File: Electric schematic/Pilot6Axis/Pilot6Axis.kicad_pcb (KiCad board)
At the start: 2 copper layers, 75.8 x 53.8 mm, 63 parts, among them IC1 ESP32-WROOM-32U, IC2 LM27313XMFX_NOPB, J1 BTN1, J10 Power switch, J11 TP4056, J12 OLED, J13 USB_C_Receptacle_USB2.0_16P, J14 BTN9, J15 BTN11, J16 BTN10, J2 BTN2, J3 BTN3, J4 BTN4, J5 BTN5, J6 BTN6, J7 BTN7, J8 BTN8, J9 BAT, Q1 Q_NPN_EBC, Q2 Q_NPN_EBC, SW1 SW_Push, SW2 SW_Push, U1 JOYSTICK1, U2 JOYSTICK2, U3 AMS1117-3.3, U4 USBLC6-2SC6, U5 CP2102N-Axx-xQFN28

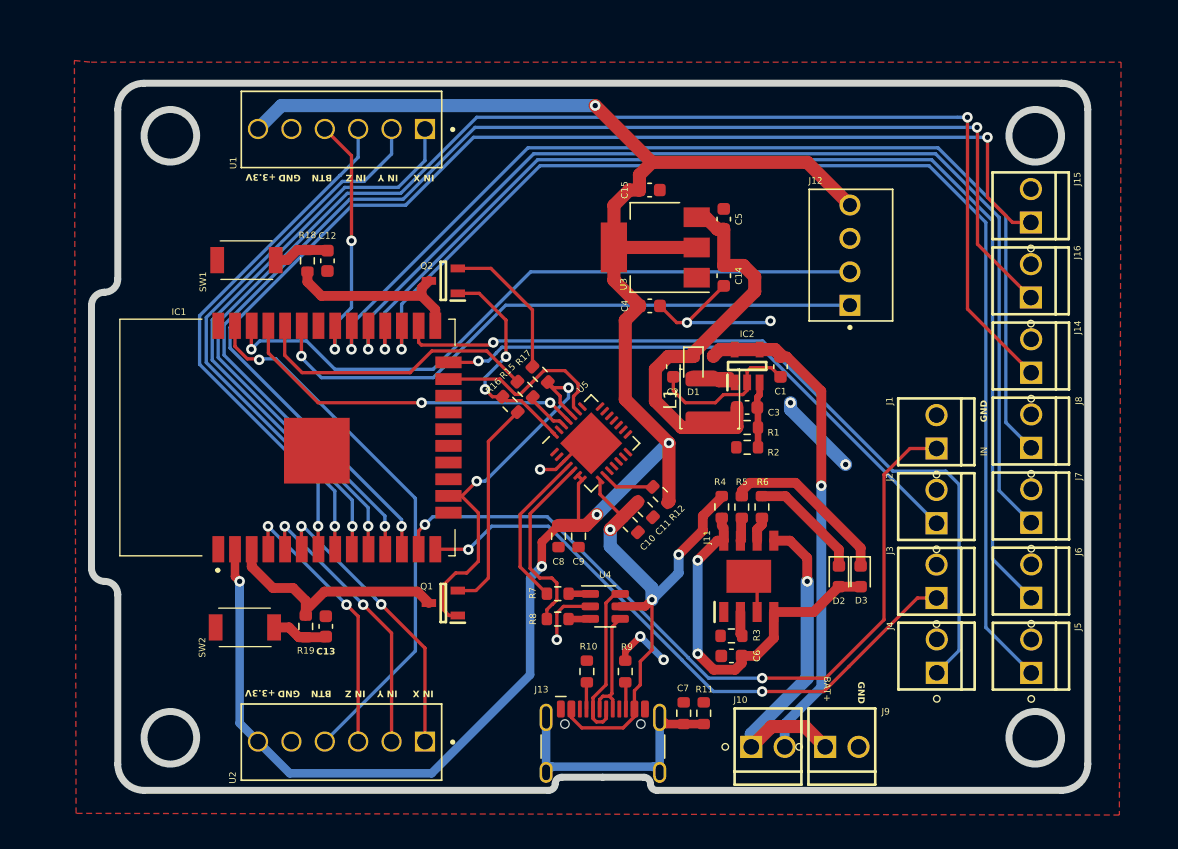
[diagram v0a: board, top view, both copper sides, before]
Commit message: Update pilot PCB versin 1.0
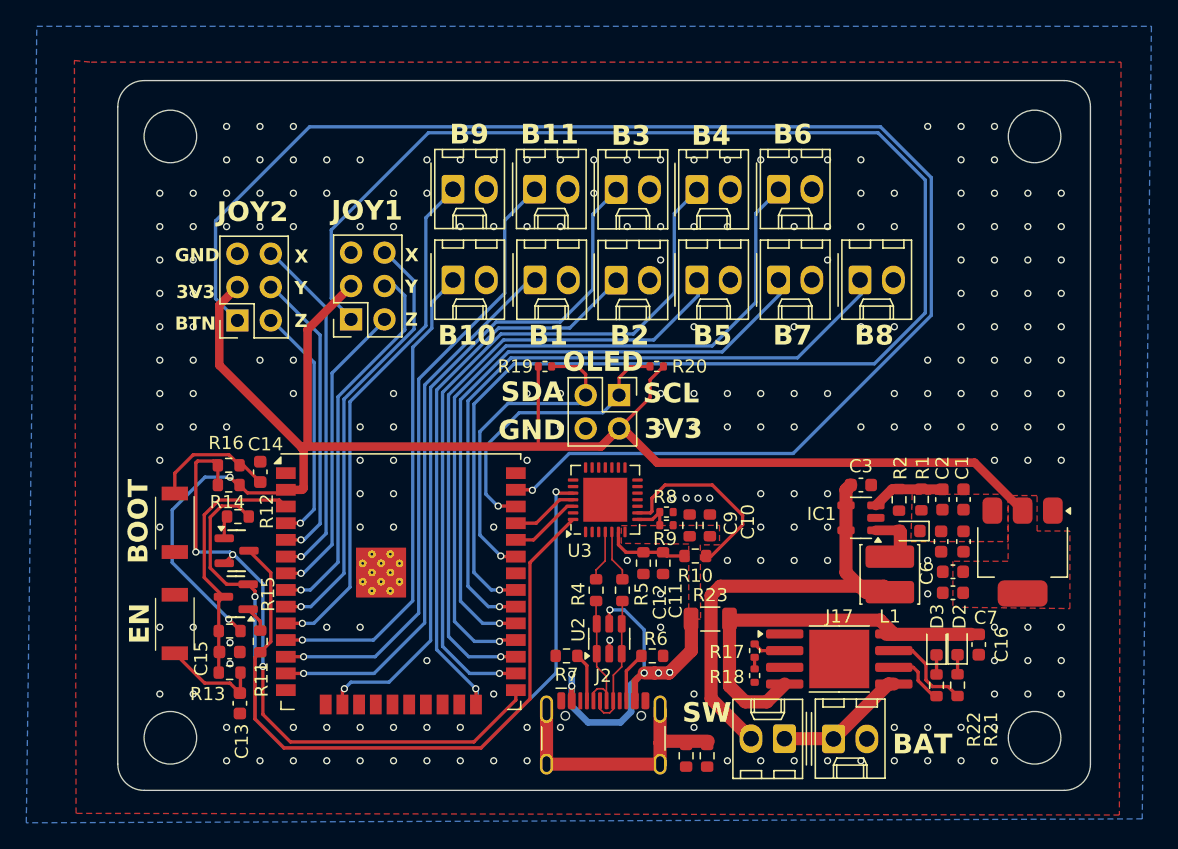
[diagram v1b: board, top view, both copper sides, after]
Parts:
- removed IC2: LM27313XMFX_NOPB, KLM27313XMF_NOPB:SOT95P280X145-5N
- removed J4: BTN4, molex-2pin:HDRV2W64P254_1X2_580X508X1170P
- removed Q2: Q_NPN_EBC, S8050:SOT95P240X115-3N
- removed U5: CP2102N-Axx-xQFN28, Package_DFN_QFN:QFN-28-1EP_5x5mm_P0.5mm_EP3.35x3.35mm
- added C16: 10uF, Capacitor_SMD:C_0603_1608Metric, F.Cu at (180.6, 114.5)
- added J17: TP4056, Package_SO:SOP-8-1EP_4.57x4.57mm_P1.27mm_EP4.57x4.45mm, F.Cu at (169.9, 115.6)
- added J18: BAT, Connector_Molex:Molex_KK-254_AE-6410-02A_1x02_P2.54mm_Vertical, F.Cu at (169.5, 121.7)
- added J19: Conn_02x03_Odd_Even, Connector_PinSocket_2.54mm:PinSocket_2x03_P2.54mm_Vertical, F.Cu at (132.8, 89.8)
- added Q3: S9014, PCM_JLCPCB:Q_SOT-23, F.Cu at (124.0, 110.9)
- added R13: 470R, Resistor_SMD:R_0603_1608Metric, F.Cu at (123.6, 116.7)
- added R14: 470R, Resistor_SMD:R_0603_1608Metric, F.Cu at (123.5, 100.9)
- added R20: 4k7, Resistor_SMD:R_0402_1005Metric, F.Cu at (156.1, 93.4)
- added R21: 1k, Resistor_SMD:R_0603_1608Metric, F.Cu at (178.9, 117.6)
- added R22: 1k, Resistor_SMD:R_0603_1608Metric, F.Cu at (177.3, 117.6)
- added R23: 0.2, Resistor_SMD:R_1206_3216Metric, F.Cu at (160.1, 112.6)
- C1: value 2.2uF -> 4.7uF
- C10: value 10uF -> 100n
- C11: value 0.1uF -> 100n
- C12: value 1nF -> 10u; footprint Capacitor_SMD:C_0603_1608Metric -> Resistor_SMD:R_0603_1608Metric
- C14, C15: value 100nF -> 1nF
- C2: value 4.7uF -> 220pF
- C3: value 220pF -> 2.2uF
- C4: value 1nF -> 100nF
- C6: value 10uF -> 1nF
- C7: value 10nF -> 100nF; footprint Resistor_SMD:R_0603_1608Metric -> Capacitor_SMD:C_0603_1608Metric
- C8: value 10uF -> 10nF
- C9: value 0.1uF -> 4.7u
- IC1: value ESP32-WROOM-32U -> LM27313XMFX_NOPB; footprint ESP32-WROOM-32U:ESP32WROOM32D -> Package_TO_SOT_SMD:SOT-23-5
- J1: value BTN1 -> Power switch; footprint molex-2pin:HDRV2W64P254_1X2_580X508X1170P -> Connector_Molex:Molex_KK-254_AE-6410-02A_1x02_P2.54mm_Vertical
- J10: value Power switch -> BTN5; footprint molex-2pin:HDRV2W64P254_1X2_580X508X1170P -> Connector_Molex:Molex_KK-254_AE-6410-02A_1x02_P2.54mm_Vertical
- J11: value TP4056 -> BTN6; footprint TP4056:SOIC127P600X175-9N -> Connector_Molex:Molex_KK-254_AE-6410-02A_1x02_P2.54mm_Vertical
- J12: value OLED -> BTN7; footprint molex-4pin:MOLEX_22232041 -> Connector_Molex:Molex_KK-254_AE-6410-02A_1x02_P2.54mm_Vertical
- J13: value USB_C_Receptacle_USB2.0_16P -> BTN8; footprint Connector_USB:USB_C_Receptacle_HCTL_HC-TYPE-C-16P-01A -> Connector_Molex:Molex_KK-254_AE-6410-02A_1x02_P2.54mm_Vertical
- J14: footprint molex-2pin:HDRV2W64P254_1X2_580X508X1170P -> Connector_Molex:Molex_KK-254_AE-6410-02A_1x02_P2.54mm_Vertical
- J15: value BTN11 -> BTN10; footprint molex-2pin:HDRV2W64P254_1X2_580X508X1170P -> Connector_Molex:Molex_KK-254_AE-6410-02A_1x02_P2.54mm_Vertical
- J16: value BTN10 -> BTN11; footprint molex-2pin:HDRV2W64P254_1X2_580X508X1170P -> Connector_Molex:Molex_KK-254_AE-6410-02A_1x02_P2.54mm_Vertical
- J2: value BTN2 -> USB_C_Receptacle_USB2.0_16P; footprint molex-2pin:HDRV2W64P254_1X2_580X508X1170P -> Connector_USB:USB_C_Receptacle_HCTL_HC-TYPE-C-16P-01A
- J3: value BTN3 -> Conn_02x03_Odd_Even; footprint molex-2pin:HDRV2W64P254_1X2_580X508X1170P -> Connector_PinSocket_2.54mm:PinSocket_2x03_P2.54mm_Vertical
- J5: value BTN5 -> Oled; footprint molex-2pin:HDRV2W64P254_1X2_580X508X1170P -> Connector_PinSocket_2.54mm:PinSocket_2x02_P2.54mm_Vertical
- J6: value BTN6 -> BTN1; footprint molex-2pin:HDRV2W64P254_1X2_580X508X1170P -> Connector_Molex:Molex_KK-254_AE-6410-02A_1x02_P2.54mm_Vertical
- J7: value BTN7 -> BTN2; footprint molex-2pin:HDRV2W64P254_1X2_580X508X1170P -> Connector_Molex:Molex_KK-254_AE-6410-02A_1x02_P2.54mm_Vertical
- J8: value BTN8 -> BTN3; footprint molex-2pin:HDRV2W64P254_1X2_580X508X1170P -> Connector_Molex:Molex_KK-254_AE-6410-02A_1x02_P2.54mm_Vertical
- J9: value BAT -> BTN4; footprint molex-2pin:HDRV2W64P254_1X2_580X508X1170P -> Connector_Molex:Molex_KK-254_AE-6410-02A_1x02_P2.54mm_Vertical
- L1: footprint Inductor_SMD:L_APV_ANR4010 -> Inductor_SMD:L_Cenker_CKCS4018
- Q1: value Q_NPN_EBC -> S9014; footprint S8050:SOT95P240X115-3N -> PCM_JLCPCB:Q_SOT-23
- R10: value 5k1 -> 1k
- R11: value 33k -> 13.3k
- R12: value 1k -> 13.3k
- R15: value 470R -> 13.3k
- R17: value 13.3k -> 1.5k; footprint Resistor_SMD:R_0603_1608Metric -> Resistor_SMD:R_0402_1005Metric
- R18: value 470R -> 1.5k; footprint Resistor_SMD:R_0603_1608Metric -> Resistor_SMD:R_0402_1005Metric
- R19: value 470R -> 4k7; footprint Resistor_SMD:R_0603_1608Metric -> Resistor_SMD:R_0402_1005Metric
- R3: value 1.2k -> 33k
- R4: value 0.5 -> 22R
- R5: value 1k -> 22R
- R6: value 1k -> 5k1
- R7: value 22R -> 5k1
- R8: value 22R -> 22k; footprint Resistor_SMD:R_0603_1608Metric -> Resistor_SMD:R_0402_1005Metric
- R9: value 5k1 -> 43k; footprint Resistor_SMD:R_0603_1608Metric -> Resistor_SMD:R_0402_1005Metric
- SW1, SW2: footprint TS-1088R-02026:TS1088R02026 -> parts:TS1088R02026
- U1: value JOYSTICK1 -> AMS1117-3.3; footprint molex-6pin:MOLEX_22-27-2061 -> Package_TO_SOT_SMD:SOT-223-3_TabPin2
- U2: value JOYSTICK2 -> USBLC6-2SC6; footprint molex-6pin:MOLEX_22-27-2061 -> Package_TO_SOT_SMD:SOT-23-6
- U3: value AMS1117-3.3 -> CP2102N-Axx-xQFN28; footprint Package_TO_SOT_SMD:SOT-223-3_TabPin2 -> Package_DFN_QFN:QFN-28-1EP_5x5mm_P0.5mm_EP3.35x3.35mm
- U4: value USBLC6-2SC6 -> ESP32-WROOM-32U; footprint Package_TO_SOT_SMD:SOT-23-6 -> RF_Module:ESP32-WROOM-32U
- moved J3 56.8 mm to (124.2, 89.9), turned to 180 degrees
- moved U1 55.7 mm to (183.9, 107.5), turned to -90 degrees
- moved C15 47.5 mm to (123.6, 115.1)
- moved R18 46.4 mm to (163.5, 116.9)
- moved J14 45.8 mm to (140.6, 79.9), turned to 0 degrees
- moved J15 44.3 mm to (140.6, 86.8), turned to 0 degrees
- moved J6 44.1 mm to (146.8, 86.8), turned to 0 degrees
- moved J9 43.8 mm to (159.1, 79.9)
- moved IC1 43.8 mm to (171.6, 104.9), turned to 180 degrees
- moved J13 41.3 mm to (171.5, 86.8)
- moved J16 38.4 mm to (146.8, 79.9), turned to 0 degrees
- moved C14 38.3 mm to (125.9, 101.4)
- moved J5 37.1 mm to (153.2, 95.6), turned to 0 degrees
- moved J8 36.5 mm to (153.0, 79.9), turned to 0 degrees
- moved J7 35.9 mm to (153.0, 86.8), turned to 0 degrees
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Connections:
- C1 pad 1: Net-(IC2-VIN) -> +5V
- C10 pad 1: VCC -> /CHARGER/VBUS
- C11 pad 1: VCC -> /USB/3.3V_USB
- C12 pad 1: GND -> /USB/3.3V_USB
- C12 pad 2: Net-(C12-Pad2) -> GND
- C13 pad 1: GND -> Net-(C13-Pad1)
- C13 pad 2: Net-(C13-Pad2) -> GND
- C14 pad 1: +5V -> GND
- C14 pad 2: GND -> Net-(C14-Pad2)
- C15 pad 1: +3.3V -> /MCU/EN
- C2 pad 1: +5V -> Net-(IC1-FB)
- C2 pad 2: GND -> +5V
- C3 pad 1: Net-(IC2-FB) -> /Power/BAT+
- C3 pad 2: +5V -> GND
- C4 pad 1: +3.3V -> +5V
- C6 pad 1: GND -> +3.3V
- C6 pad 2: Net-(D2-A) -> GND
- C7 pad 1: Net-(J13-SHIELD) -> +3.3V
- C8 pad 1: +3.3V -> Net-(J2-SHIELD)
- C9 pad 1: +3.3V -> /CHARGER/VBUS
- D2 pad 2: Net-(D2-A) -> /CHARGER/VCC4
- D3 pad 2: Net-(D2-A) -> /CHARGER/VCC4
- IC1 pad 1: GND -> Net-(D1-A)
- IC1 pad 2: +3.3V -> GND
- IC1 pad 3: /EN -> Net-(IC1-FB)
- IC1 pad 4: /JOYSTICK2_Z -> /Power/BAT+
- IC1 pad 5: /JOYSTICK2_Y -> /Power/BAT+
- J1 pad 1: /BTN1 -> /CHARGER/BAT+
- J1 pad 2: GND -> /Power/BAT+
- J10 pad 1: /BAT+ -> /MCU/BTN5
- J10 pad 2: Net-(IC2-VIN) -> GND
- J11 pad 1: GND -> /MCU/BTN6
- J11 pad 2: Net-(J11-PROG2) -> GND
- J12 pad 1: /SDA -> /MCU/BTN7
- J12 pad 2: /SCL -> GND
- J14 pad 1: /BTN9 -> /MCU/BTN9
- J15 pad 1: /BTN11 -> /MCU/BTN10
- J16 pad 1: /BTN10 -> /MCU/BTN11
- J3 pad 1: /BTN3 -> /MCU/JOYSTICK2_BTN
- J3 pad 2: GND -> /MCU/JOYSTICK2_Z
- J5 pad 1: /BTN5 -> /MCU/SCL
- J5 pad 2: GND -> /MCU/SDA
- J6 pad 1: /BTN6 -> /MCU/BTN1
- J7 pad 1: /BTN7 -> /MCU/BTN2
- J8 pad 1: /BTN8 -> /MCU/BTN3
- J9 pad 1: /BAT+ -> /MCU/BTN4
- L1 pad 2: Net-(IC2-VIN) -> /Power/BAT+
- Q1 pad 1: /RST -> Net-(Q1-B)
- Q1 pad 2: Net-(Q1-B) -> /MCU/IO0
- Q1 pad 3: /EN -> /USB/DTR
- R1 pad 2: Net-(IC2-FB) -> Net-(IC1-FB)
- R10 pad 1: Net-(J13-CC1) -> /USB/3.3V_USB
- R10 pad 2: GND -> Net-(U3-~{RST})
- R11 pad 1: Net-(J13-SHIELD) -> /USB/DTR
- R11 pad 2: GND -> Net-(Q3-B)
- R12 pad 1: +3.3V -> /USB/RTS
- R12 pad 2: Net-(U5-~{RST}) -> Net-(Q1-B)
- R15 pad 1: Net-(U5-TXD) -> /MCU/EN
- R15 pad 2: /TXD -> +3.3V
- R16 pad 1: /DTR -> /MCU/IO0
- R16 pad 2: Net-(Q1-B) -> +3.3V
- R17 pad 1: /RST -> /CHARGER/PROG2
- R17 pad 2: Net-(Q2-B) -> Net-(R17-Pad2)
- R18 pad 1: Net-(C12-Pad2) -> Net-(R17-Pad2)
- R18 pad 2: /IO0 -> GND
- R19 pad 1: Net-(C13-Pad2) -> /MCU/SDA
- R19 pad 2: /EN -> +3.3V
- R2 pad 2: Net-(IC2-FB) -> Net-(IC1-FB)
- R3 pad 1: Net-(J11-PROG2) -> Net-(J2-SHIELD)
- R4 pad 1: VCC -> /USB/USB_CONN_D-
- R4 pad 2: Net-(D2-A) -> /USB/D+
- R5 pad 1: Net-(D3-K) -> /USB/USB_CONN_D+
- R5 pad 2: Net-(J11-~{CHRG}) -> /USB/D-
- R6 pad 1: Net-(D2-K) -> Net-(J2-CC2)
- R6 pad 2: Net-(J11-~{STDBY}) -> GND
- R7 pad 1: Net-(R7-Pad1) -> Net-(J2-CC1)
- R7 pad 2: /D+ -> GND
- R8 pad 1: Net-(R8-Pad1) -> Net-(U3-VBUS)
- R8 pad 2: /D- -> /CHARGER/VBUS
- R9 pad 1: Net-(J13-CC2) -> GND
- R9 pad 2: GND -> Net-(U3-VBUS)
- SW1 pad 2: Net-(C12-Pad2) -> Net-(C13-Pad1)
- SW2 pad 2: Net-(C13-Pad2) -> Net-(C14-Pad2)
- U1 pad 1: /JOYSTICK1_X -> GND
- U1 pad 2: /JOYSTICK1_Y -> +3.3V
- U1 pad 3: /JOYSTICK1_Z -> +5V
- U2 pad 1: /JOYSTICK2_X -> /USB/USB_CONN_D-
- U2 pad 2: /JOYSTICK2_Y -> GND
- U2 pad 3: /JOYSTICK2_Z -> /USB/USB_CONN_D+
- U2 pad 4: /JOYSTICK2_BTN -> /USB/USB_CONN_D+
- U2 pad 5: GND -> /CHARGER/VBUS
- U2 pad 6: +3.3V -> /USB/USB_CONN_D-
- U3 pad 1: GND -> unconnected-(U3-~{DCD}-Pad1)
- U3 pad 2: +3.3V -> unconnected-(U3-~{RI}/CLK-Pad2)
- U3 pad 3: +5V -> GND
- U4 pad 1: Net-(R7-Pad1) -> GND
- U4 pad 2: GND -> +3.3V
- U4 pad 3: Net-(R8-Pad1) -> /MCU/EN
- U4 pad 4: /USB_CONN_D+ -> /MCU/JOYSTICK2_Z
- U4 pad 5: VCC -> /MCU/JOYSTICK2_Y
- U4 pad 6: /USB_CONN_D- -> /MCU/JOYSTICK2_X
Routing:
- net /MCU/JOYSTICK1_BTN: track 0.00 -> 121.1 mm, vias 0 -> 1
- net /MCU/JOYSTICK2_BTN: track 0.00 -> 114.9 mm, vias 0 -> 1
- net /BTN9: track 107.2 -> 0.00 mm, vias 2 -> 0
- net /BTN10: track 100.3 -> 0.00 mm, vias 2 -> 0
- net /BTN11: track 94.9 -> 0.00 mm, vias 2 -> 0
- net /BTN5: track 91.5 -> 0.00 mm, vias 1 -> 0
- net /BTN6: track 87.5 -> 0.00 mm, vias 1 -> 0
- net /BTN7: track 83.5 -> 0.00 mm, vias 1 -> 0
- net /BTN8: track 79.6 -> 0.00 mm, vias 1 -> 0
- net /USB/RTS: track 0.00 -> 62.6 mm, vias 0 -> 2
- net /BTN4: track 62.1 -> 0.00 mm, vias 1 -> 0
- net /BTN1: track 60.2 -> 0.00 mm, vias 2 -> 0
- net /MCU/BTN6: track 0.00 -> 57.7 mm, vias 0 -> 1
- net /MCU/BTN4: track 0.00 -> 55.1 mm, vias 0 -> 1
- net /MCU/BTN8: track 0.00 -> 52.8 mm, vias 0 -> 1
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- added copper zone on F.Cu, net +3.3V
- added copper zone on F.Cu, net +5V
- added copper zone on F.Cu, net /CHARGER/VBUS
- added copper zone on B.Cu, net GND
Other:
- board size 75.8 x 53.8 mm -> 74 x 54 mm
- board text added: "3V3"
- board text added: "B1"
- board text added: "B10"
- board text added: "B11"
- board text added: "B2"
- board text added: "B3"
- board text added: "B4"
- board text added: "B5"
- board text added: "B6"
- board text added: "B7"
- board text added: "B8"
- board text added: "B9"
- board text added: "BAT"
- board text added: "BOOT"
- board text added: "EN"
- board text added: "JOY1"
- board text added: "JOY2"
- board text added: "OLED"
- board text added: "SCL"
- board text added: "SDA"
- board text added: "SW"
- board text added: "VBAT"
- board text added: "X"
- board text added: "Y"
- board text added: "Z"
- board text removed: "+3.3V"
- board text removed: "BAT+"
- board text removed: "IN"
- board text removed: "IN X"
- board text removed: "IN Y"
- board text removed: "IN Z"
